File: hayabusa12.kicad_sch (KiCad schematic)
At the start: 32 parts, among them J1 USB_C_Receptacle_USB2.0, SW1 SW_Push, SW10 MX_SW_HS, SW11 MX_SW_HS, SW12 MX_SW_HS, SW13 MX_SW_HS, SW2 MX_SW_HS, SW3 MX_SW_HS, SW4 MX_SW_HS, SW5 MX_SW_HS, SW6 MX_SW_HS, SW7 MX_SW_HS, SW8 MX_SW_HS, SW9 MX_SW_HS, U1 ATmega32U4-AU, U2 SRV05-4, Y1 16MHz

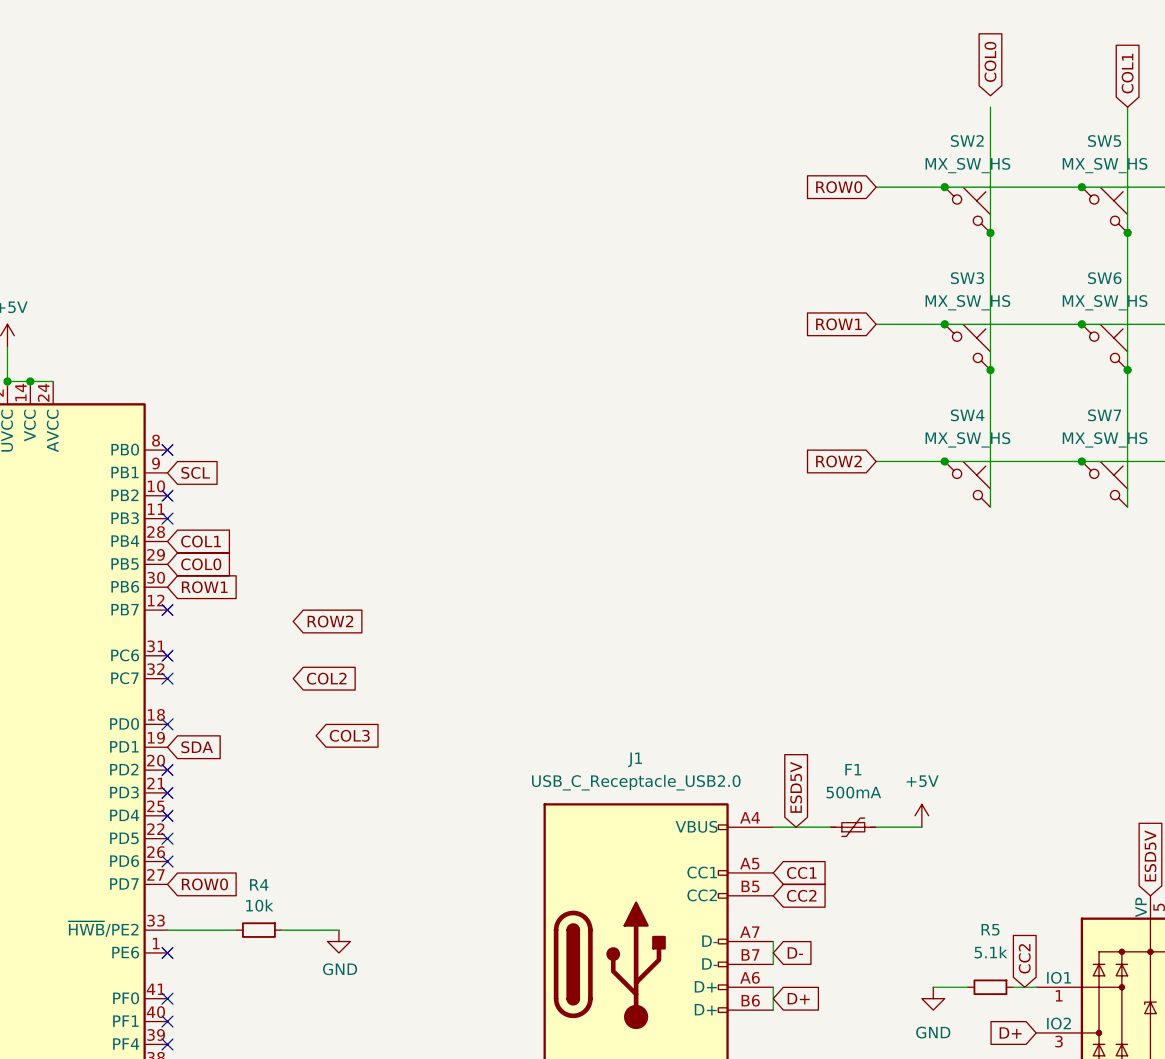
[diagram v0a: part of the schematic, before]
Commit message: routing
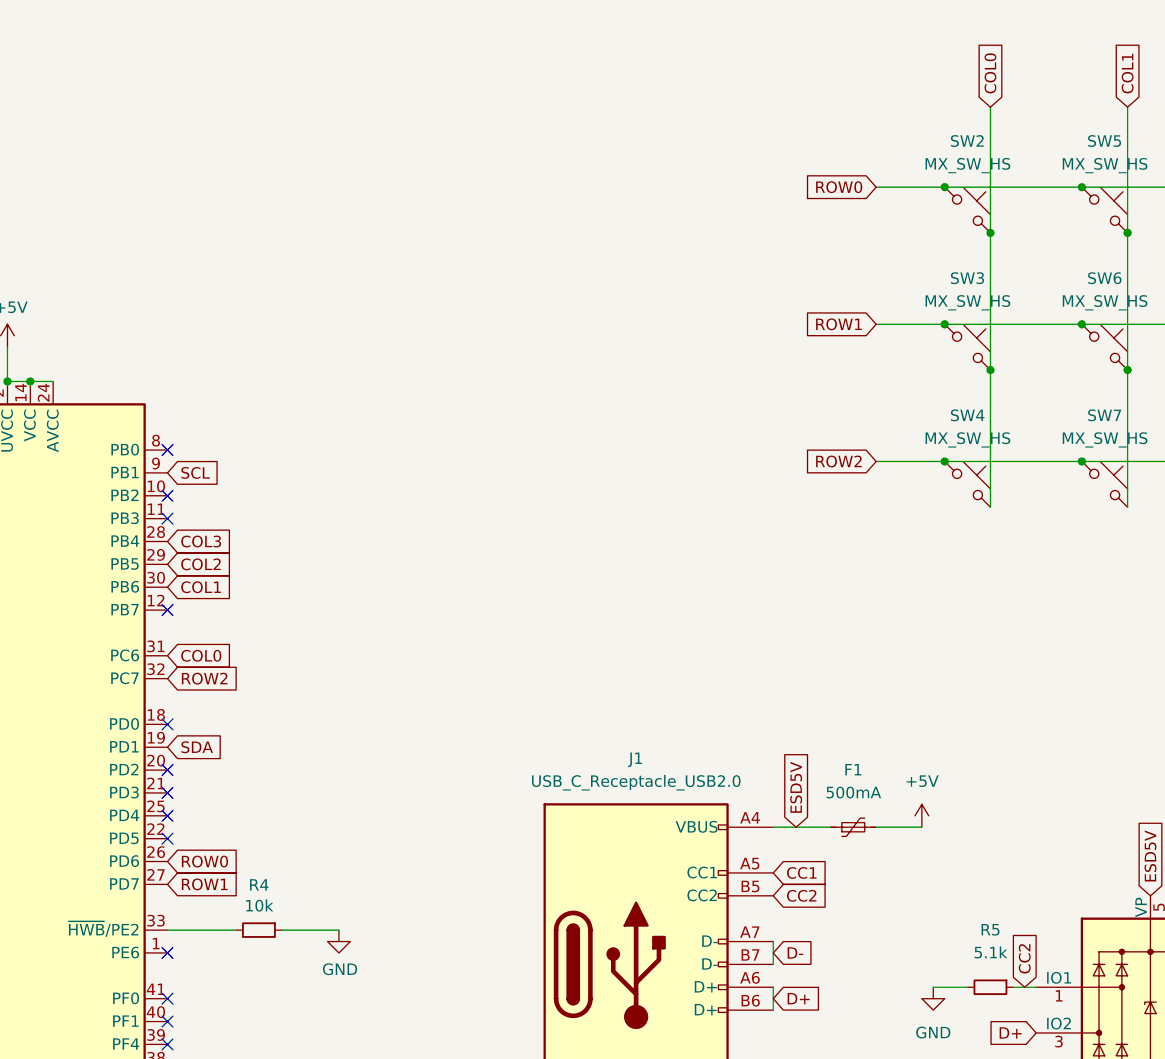
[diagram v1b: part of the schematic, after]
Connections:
- net COL0: now also SW2.2, SW3.2, SW4.2, U1.31 (PC6); no longer U1.29 (PB5)
- net COL1: now also U1.30 (PB6); no longer U1.28 (PB4)
- net COL2: now also U1.29 (PB5)
- net COL3: now also U1.28 (PB4)
- net ROW0: now also U1.26 (PD6); no longer U1.27 (PD7)
- net ROW1: now also U1.27 (PD7); no longer U1.30 (PB6)
- net ROW2: now also U1.32 (PC7)
- no-connect marks 22 -> 19
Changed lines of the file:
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@@
   (no_connect (at 93.98 101.6))
   (no_connect (at 93.98 134.62))
-  (no_connect (at 93.98 91.44))
-  (no_connect (at 93.98 111.76))
   (no_connect (at 93.98 104.14))
   (no_connect (at 161.29 135.89))
@@
   (no_connect (at 63.5 81.28))
   (no_connect (at 93.98 132.08))
-  (no_connect (at 93.98 88.9))
   (wire (pts (xy 232.41 109.22) (xy 237.49 109.22))
     (stroke (width 0) (type default) (color 0 0 0 0))
@@
     (stroke (width 0) (type default) (color 0 0 0 0))
   )
+  (wire (pts (xy 210.82 36.83) (xy 226.06 36.83))
+    (stroke (width 0) (type default) (color 0 0 0 0))
+  )
   (wire (pts (xy 36.83 68.58) (xy 36.83 71.12))
     (stroke (width 0) (type default) (color 0 0 0 0))
@@
   )
   (wire (pts (xy 31.75 68.58) (xy 31.75 78.74))
-    (stroke (width 0) (type default) (color 0 0 0 0))
-  )
-  (wire (pts (xy 210.82 36.83) (xy 226.06 36.83))
     (stroke (width 0) (type default) (color 0 0 0 0))
   )
@@
     )
   )
-  (global_label "ROW0" (shape input) (at 93.98 114.3 0) (fields_autoplaced)
-    (effects (font (size 1.27 1.27)) (justify left))
-    (property "Intersheet References" "${INTERSHEET_REFS}" (id 0) (at 1.27 7.62 0)
+  (global_label "ROW0" (shape input) (at 93.98 111.76 0) (fields_autoplaced)
+    (effects (font (size 1.27 1.27)) (justify left))
+    (property "Intersheet References" "${INTERSHEET_REFS}" (id 0) (at 1.27 5.08 0)
       (effects (font (size 1.27 1.27)) hide)
     )
@@
     )
   )
-  (global_label "COL1" (shape input) (at 93.98 76.2 0) (fields_autoplaced)
-    (effects (font (size 1.27 1.27)) (justify left))
-    (property "Intersheet References" "${INTERSHEET_REFS}" (id 0) (at 1.27 7.62 0)
+  (global_label "COL1" (shape input) (at 93.98 81.28 0) (fields_autoplaced)
+    (effects (font (size 1.27 1.27)) (justify left))
+    (property "Intersheet References" "${INTERSHEET_REFS}" (id 0) (at 1.27 12.7 0)
       (effects (font (size 1.27 1.27)) hide)
     )
@@
     )
   )
-  (global_label "COL2" (shape input) (at 107.95 91.44 0) (fields_autoplaced)
-    (effects (font (size 1.27 1.27)) (justify left))
-    (property "Intersheet References" "${INTERSHEET_REFS}" (id 0) (at 115.2012 91.3606 0)
+  (global_label "COL2" (shape input) (at 93.98 78.74 0) (fields_autoplaced)
+    (effects (font (size 1.27 1.27)) (justify left))
+    (property "Intersheet References" "${INTERSHEET_REFS}" (id 0) (at 101.2312 78.6606 0)
       (effects (font (size 1.27 1.27)) (justify left) hide)
     )
@@
     )
   )
-  (global_label "ROW1" (shape input) (at 93.98 81.28 0) (fields_autoplaced)
-    (effects (font (size 1.27 1.27)) (justify left))
-    (property "Intersheet References" "${INTERSHEET_REFS}" (id 0) (at 1.27 7.62 0)
-      (effects (font (size 1.27 1.27)) hide)
-    )
-  )
-  (global_label "COL0" (shape input) (at 93.98 78.74 0) (fields_autoplaced)
-    (effects (font (size 1.27 1.27)) (justify left))
-    (property "Intersheet References" "${INTERSHEET_REFS}" (id 0) (at 1.27 7.62 0)
+  (global_label "ROW1" (shape input) (at 93.98 114.3 0) (fields_autoplaced)
+    (effects (font (size 1.27 1.27)) (justify left))
+    (property "Intersheet References" "${INTERSHEET_REFS}" (id 0) (at 1.27 40.64 0)
+      (effects (font (size 1.27 1.27)) hide)
+    )
+  )
+  (global_label "COL0" (shape input) (at 93.98 88.9 0) (fields_autoplaced)
+    (effects (font (size 1.27 1.27)) (justify left))
+    (property "Intersheet References" "${INTERSHEET_REFS}" (id 0) (at 1.27 17.78 0)
       (effects (font (size 1.27 1.27)) hide)
     )
@@
     )
   )
-  (global_label "COL3" (shape input) (at 110.49 97.79 0) (fields_autoplaced)
-    (effects (font (size 1.27 1.27)) (justify left))
-    (property "Intersheet References" "${INTERSHEET_REFS}" (id 0) (at 117.7412 97.7106 0)
+  (global_label "COL3" (shape input) (at 93.98 76.2 0) (fields_autoplaced)
+    (effects (font (size 1.27 1.27)) (justify left))
+    (property "Intersheet References" "${INTERSHEET_REFS}" (id 0) (at 101.2312 76.1206 0)
       (effects (font (size 1.27 1.27)) (justify left) hide)
     )
@@
     )
   )
-  (global_label "COL0" (shape input) (at 185.42 26.67 90) (fields_autoplaced)
-    (effects (font (size 1.27 1.27)) (justify left))
-    (property "Intersheet References" "${INTERSHEET_REFS}" (id 0) (at 30.48 -39.37 0)
+  (global_label "COL0" (shape input) (at 185.42 27.94 90) (fields_autoplaced)
+    (effects (font (size 1.27 1.27)) (justify left))
+    (property "Intersheet References" "${INTERSHEET_REFS}" (id 0) (at 30.48 -38.1 0)
       (effects (font (size 1.27 1.27)) hide)
     )
@@
     )
   )
-  (global_label "ROW2" (shape input) (at 107.95 85.09 0) (fields_autoplaced)
-    (effects (font (size 1.27 1.27)) (justify left))
-    (property "Intersheet References" "${INTERSHEET_REFS}" (id 0) (at 115.6245 85.0106 0)
-      (effects (font (size 1.27 1.27)) (justify left) hide)
-    )
+  (global_label "ROW2" (shape input) (at 93.98 91.44 0) (fields_autoplaced)
+    (effects (font (size 1.27 1.27)) (justify left))
+    (property "Intersheet References" "${INTERSHEET_REFS}" (id 0) (at 101.6545 91.3606 0)
+      (effects (font (size 1.27 1.27)) (justify left) hide)
+    )
